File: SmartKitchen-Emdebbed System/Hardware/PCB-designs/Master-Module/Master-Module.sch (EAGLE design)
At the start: 12 parts, among them IC2 7805DT, J1 RJ11-2L-B, J2 RJ11-2L-B, J3 RJ11-2L-B, X1 K375M

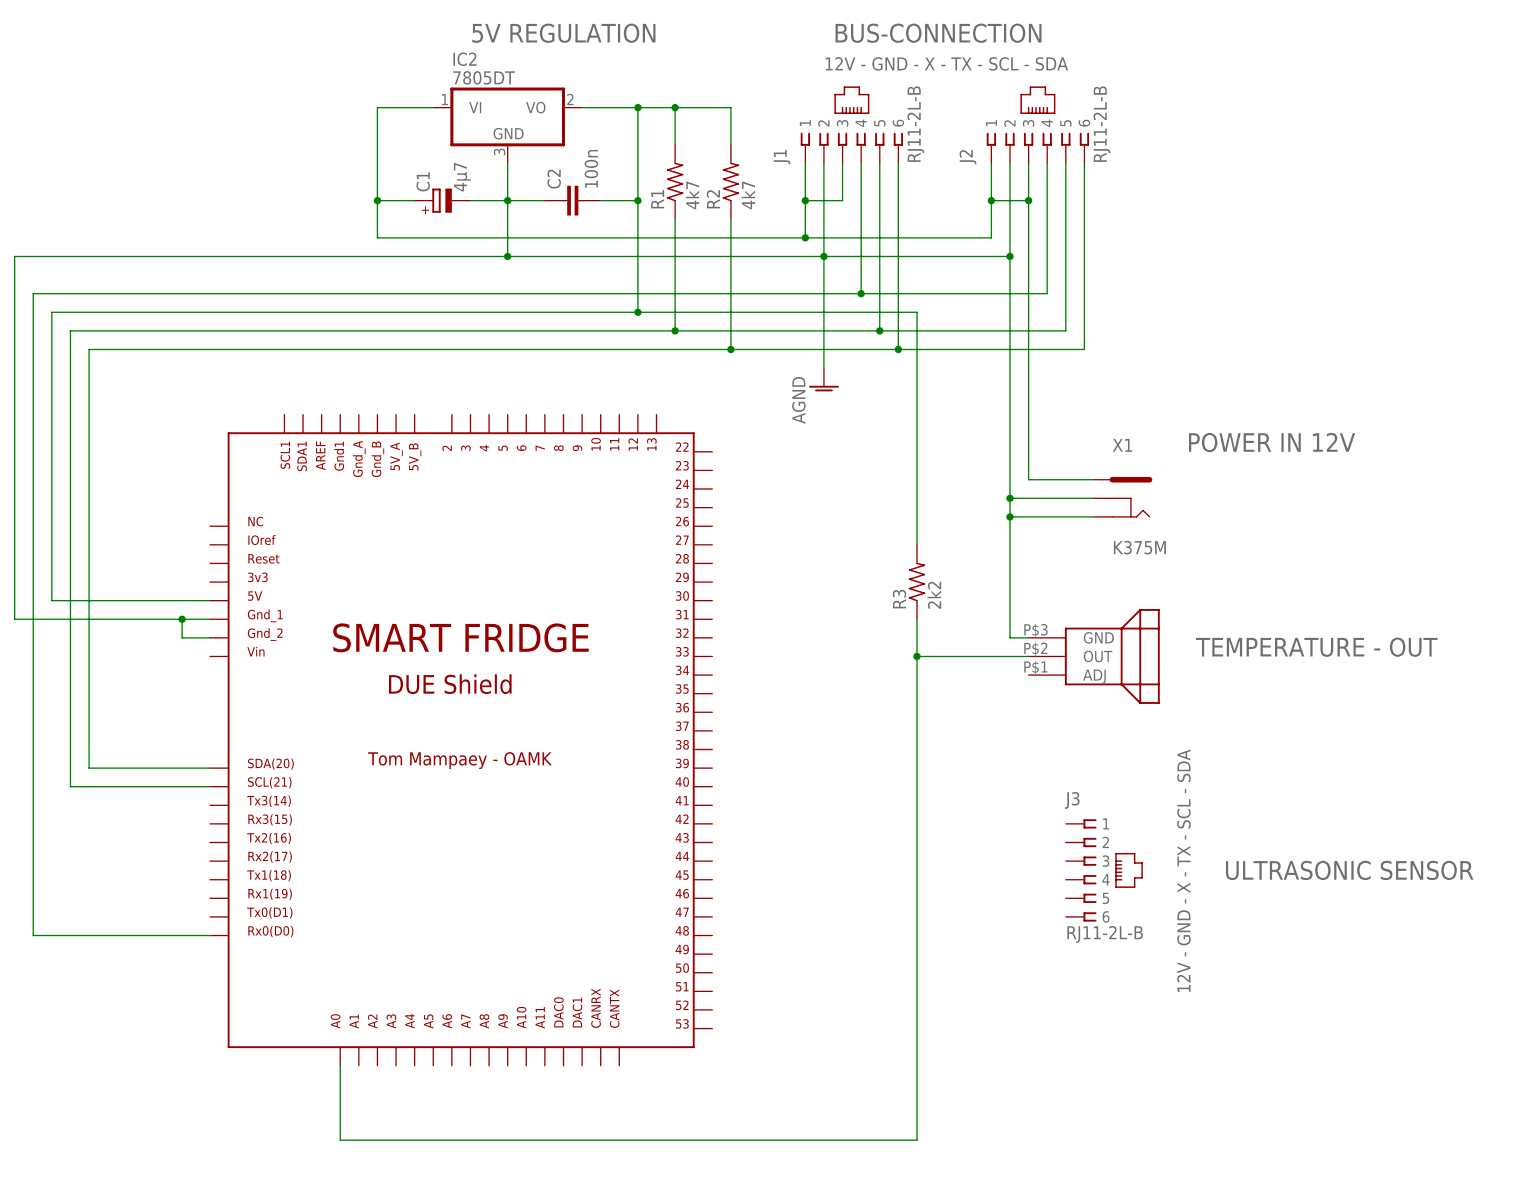
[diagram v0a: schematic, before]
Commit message: PCB shield
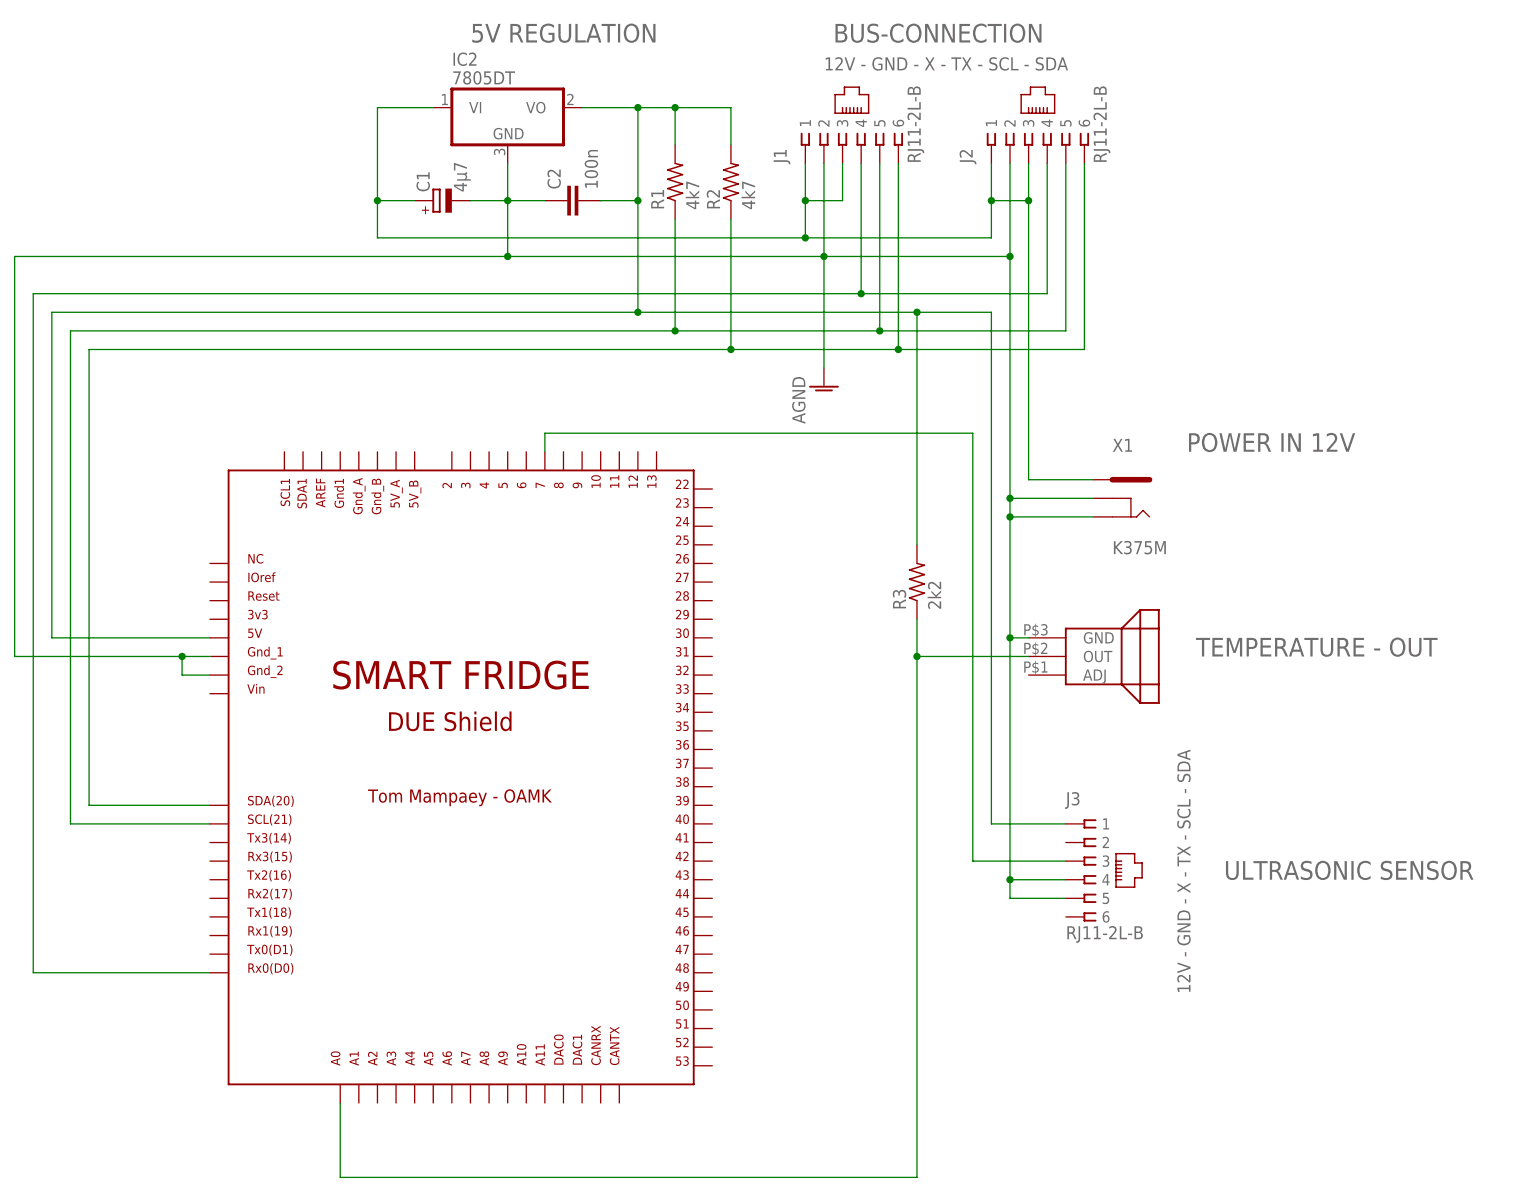
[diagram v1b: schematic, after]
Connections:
- new net N$6: J3.3, U$1.7
- net AGND: now also J3.4, J3.5
- net N$21: now also J3.1
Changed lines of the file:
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@@
 <instance part="R2" gate="G$1" x="118.11" y="182.88" rot="R90"/>
 <instance part="FRAME1" gate="G$1" x="-8.89" y="31.75"/>
-<instance part="U$1" gate="G$1" x="81.28" y="107.95"/>
+<instance part="U$1" gate="G$1" x="81.28" y="102.87"/>
 <instance part="X1" gate="G$1" x="172.72" y="139.7"/>
 <instance part="R3" gate="G$1" x="143.51" y="128.27" rot="R90"/>
@@
 <wire x1="118.11" y1="177.8" x2="118.11" y2="160.02" width="0.1524" layer="91"/>
 <junction x="118.11" y="160.02"/>
-<wire x1="30.48" y1="160.02" x2="30.48" y2="102.87" width="0.1524" layer="91"/>
-<wire x1="30.48" y1="102.87" x2="46.99" y2="102.87" width="0.1524" layer="91"/>
+<wire x1="30.48" y1="160.02" x2="30.48" y2="97.79" width="0.1524" layer="91"/>
+<wire x1="30.48" y1="97.79" x2="46.99" y2="97.79" width="0.1524" layer="91"/>
 <pinref part="U$1" gate="G$1" pin="SDA"/>
 </segment>
@@
 <wire x1="110.49" y1="177.8" x2="110.49" y2="162.56" width="0.1524" layer="91"/>
 <junction x="110.49" y="162.56"/>
-<wire x1="27.94" y1="162.56" x2="27.94" y2="100.33" width="0.1524" layer="91"/>
-<wire x1="27.94" y1="100.33" x2="46.99" y2="100.33" width="0.1524" layer="91"/>
+<wire x1="27.94" y1="162.56" x2="27.94" y2="95.25" width="0.1524" layer="91"/>
+<wire x1="27.94" y1="95.25" x2="46.99" y2="95.25" width="0.1524" layer="91"/>
 <pinref part="U$1" gate="G$1" pin="SCL"/>
 </segment>
@@
 <wire x1="118.11" y1="193.04" x2="110.49" y2="193.04" width="0.1524" layer="91"/>
 <junction x="110.49" y="193.04"/>
-<wire x1="25.4" y1="165.1" x2="25.4" y2="125.73" width="0.1524" layer="91"/>
-<wire x1="25.4" y1="125.73" x2="46.99" y2="125.73" width="0.1524" layer="91"/>
+<wire x1="25.4" y1="165.1" x2="25.4" y2="120.65" width="0.1524" layer="91"/>
+<wire x1="25.4" y1="120.65" x2="46.99" y2="120.65" width="0.1524" layer="91"/>
 <pinref part="U$1" gate="G$1" pin="5V"/>
 <junction x="105.41" y="165.1"/>
@@
 <wire x1="143.51" y1="165.1" x2="105.41" y2="165.1" width="0.1524" layer="91"/>
 <wire x1="143.51" y1="133.35" x2="143.51" y2="165.1" width="0.1524" layer="91"/>
+<pinref part="J3" gate="G$1" pin="1"/>
+<wire x1="163.83" y1="95.25" x2="153.67" y2="95.25" width="0.1524" layer="91"/>
+<wire x1="153.67" y1="95.25" x2="153.67" y2="165.1" width="0.1524" layer="91"/>
+<wire x1="153.67" y1="165.1" x2="143.51" y2="165.1" width="0.1524" layer="91"/>
+<junction x="143.51" y="165.1"/>
 </segment>
 </net>
@@
 <wire x1="135.89" y1="185.42" x2="135.89" y2="167.64" width="0.1524" layer="91"/>
 <junction x="135.89" y="167.64"/>
-<wire x1="22.86" y1="167.64" x2="22.86" y2="80.01" width="0.1524" layer="91"/>
-<wire x1="46.99" y1="80.01" x2="22.86" y2="80.01" width="0.1524" layer="91"/>
+<wire x1="22.86" y1="167.64" x2="22.86" y2="74.93" width="0.1524" layer="91"/>
+<wire x1="46.99" y1="74.93" x2="22.86" y2="74.93" width="0.1524" layer="91"/>
 <pinref part="U$1" gate="G$1" pin="RX0"/>
 </segment>
@@
 <pinref part="AGND4" gate="VR1" pin="AGND"/>
 <wire x1="130.81" y1="157.48" x2="130.81" y2="172.72" width="0.1524" layer="91"/>
-<wire x1="20.32" y1="172.72" x2="20.32" y2="123.19" width="0.1524" layer="91"/>
-<wire x1="20.32" y1="123.19" x2="43.18" y2="123.19" width="0.1524" layer="91"/>
+<wire x1="20.32" y1="172.72" x2="20.32" y2="118.11" width="0.1524" layer="91"/>
+<wire x1="20.32" y1="118.11" x2="43.18" y2="118.11" width="0.1524" layer="91"/>
 <pinref part="U$1" gate="G$1" pin="GND_1"/>
-<wire x1="43.18" y1="123.19" x2="46.99" y2="123.19" width="0.1524" layer="91"/>
+<wire x1="43.18" y1="118.11" x2="46.99" y2="118.11" width="0.1524" layer="91"/>
 <wire x1="156.21" y1="137.16" x2="156.21" y2="139.7" width="0.1524" layer="91"/>
 <junction x="156.21" y="172.72"/>
@@
 <wire x1="167.64" y1="137.16" x2="156.21" y2="137.16" width="0.1524" layer="91"/>
 <pinref part="U$1" gate="G$1" pin="GND_2"/>
-<wire x1="46.99" y1="120.65" x2="43.18" y2="120.65" width="0.1524" layer="91"/>
-<wire x1="43.18" y1="120.65" x2="43.18" y2="123.19" width="0.1524" layer="91"/>
-<junction x="43.18" y="123.19"/>
+<wire x1="46.99" y1="115.57" x2="43.18" y2="115.57" width="0.1524" layer="91"/>
+<wire x1="43.18" y1="115.57" x2="43.18" y2="118.11" width="0.1524" layer="91"/>
+<junction x="43.18" y="118.11"/>
 <wire x1="158.75" y1="120.65" x2="156.21" y2="120.65" width="0.1524" layer="91"/>
 <wire x1="156.21" y1="120.65" x2="156.21" y2="137.16" width="0.1524" layer="91"/>
 <junction x="156.21" y="137.16"/>
 <pinref part="U$2" gate="G$1" pin="GND"/>
+<pinref part="J3" gate="G$1" pin="4"/>
+<wire x1="163.83" y1="87.63" x2="156.21" y2="87.63" width="0.1524" layer="91"/>
+<wire x1="156.21" y1="87.63" x2="156.21" y2="120.65" width="0.1524" layer="91"/>
+<junction x="156.21" y="120.65"/>
+<pinref part="J3" gate="G$1" pin="5"/>
+<wire x1="163.83" y1="85.09" x2="156.21" y2="85.09" width="0.1524" layer="91"/>
+<wire x1="156.21" y1="85.09" x2="156.21" y2="87.63" width="0.1524" layer="91"/>
+<junction x="156.21" y="87.63"/>
 </segment>
 </net>
@@
 <segment>
 <wire x1="158.75" y1="118.11" x2="143.51" y2="118.11" width="0.1524" layer="91"/>
-<wire x1="143.51" y1="118.11" x2="143.51" y2="52.07" width="0.1524" layer="91"/>
+<wire x1="143.51" y1="118.11" x2="143.51" y2="46.99" width="0.1524" layer="91"/>
 <pinref part="U$1" gate="G$1" pin="A0"/>
-<wire x1="143.51" y1="52.07" x2="64.77" y2="52.07" width="0.1524" layer="91"/>
-<wire x1="64.77" y1="52.07" x2="64.77" y2="62.23" width="0.1524" layer="91"/>
+<wire x1="143.51" y1="46.99" x2="64.77" y2="46.99" width="0.1524" layer="91"/>
+<wire x1="64.77" y1="46.99" x2="64.77" y2="57.15" width="0.1524" layer="91"/>
 <pinref part="R3" gate="G$1" pin="1"/>
 <wire x1="143.51" y1="118.11" x2="143.51" y2="123.19" width="0.1524" layer="91"/>
@@
 </segment>
 </net>
+<net name="N$6" class="0">
+<segment>
+<pinref part="J3" gate="G$1" pin="3"/>
+<wire x1="163.83" y1="90.17" x2="151.13" y2="90.17" width="0.1524" layer="91"/>
+<wire x1="151.13" y1="90.17" x2="151.13" y2="148.59" width="0.1524" layer="91"/>
+<wire x1="151.13" y1="148.59" x2="92.71" y2="148.59" width="0.1524" layer="91"/>
+<pinref part="U$1" gate="G$1" pin="7"/>
+<wire x1="92.71" y1="148.59" x2="92.71" y2="146.05" width="0.1524" layer="91"/>
+</segment>
+</net>
